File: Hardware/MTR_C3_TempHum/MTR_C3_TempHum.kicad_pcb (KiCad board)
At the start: 4 copper layers, 75 x 19 mm, 6 parts, among them IC1 ESP32-C3-MINI-1-H4, IC2 BQ25170DSGR, IC3 TLV76733DRVR, IC4 DHT22, J1 USB_C_Receptacle_USB2.0

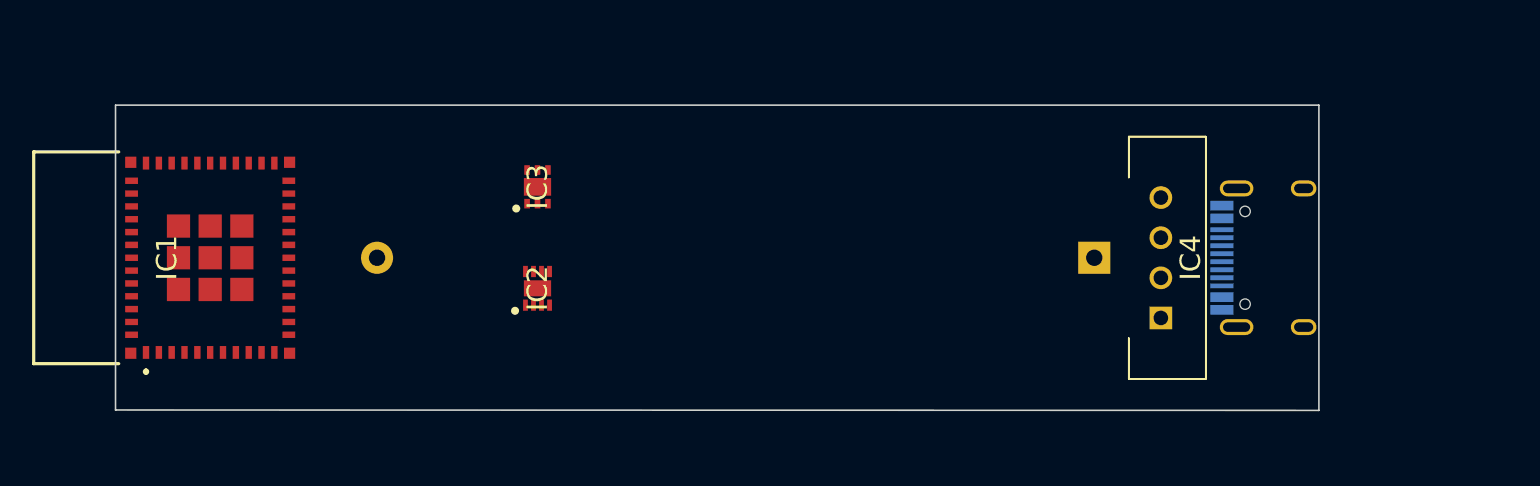
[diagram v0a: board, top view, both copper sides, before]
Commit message: REV 0.1
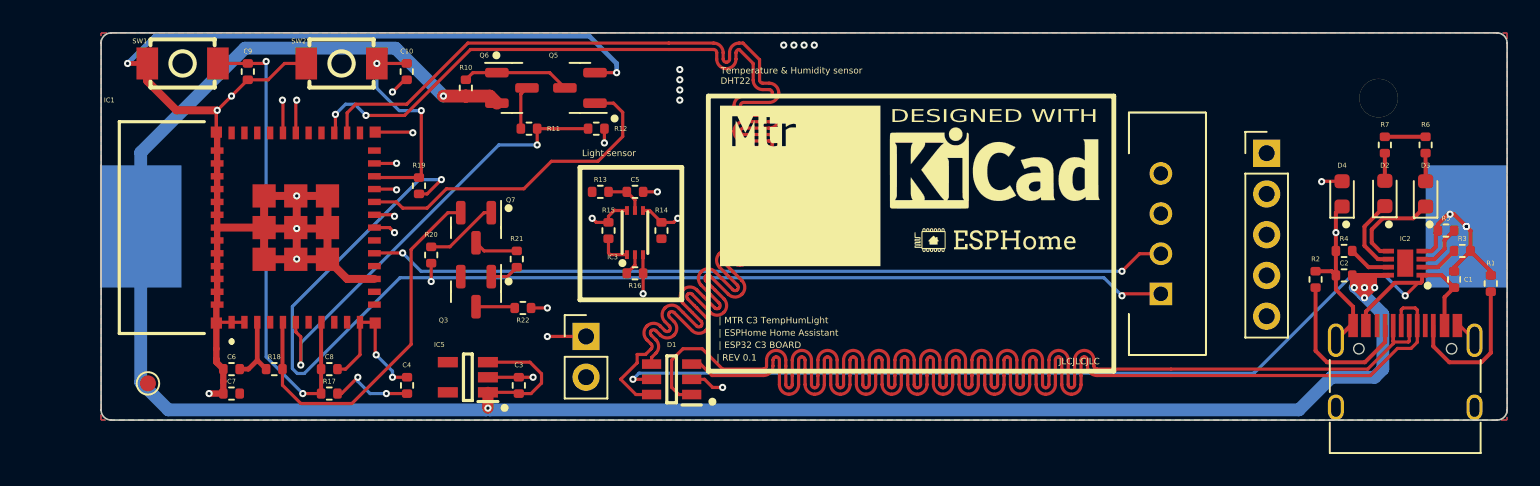
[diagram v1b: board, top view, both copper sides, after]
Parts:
- added ?: , clipboard:4e852f44-b39c-41c1-9906-6824c0cbc5c7, F.Cu at (62.7, 28.7)
- added ?: , clipboard:4e852f44-b39c-41c1-9906-6824c0cbc5c7, F.Cu at (63.2, 50.7)
- added ?: , clipboard:4e852f44-b39c-41c1-9906-6824c0cbc5c7, F.Cu at (118.4, 39.2)
- added ?: , clipboard:4e852f44-b39c-41c1-9906-6824c0cbc5c7, F.Cu at (120.9, 39.2)
- added ?: , clipboard:4e852f44-b39c-41c1-9906-6824c0cbc5c7, F.Cu at (70.1, 32.6)
- added ?: , clipboard:4e852f44-b39c-41c1-9906-6824c0cbc5c7, F.Cu at (76.2, 50.3)
- added ?: , clipboard:4e852f44-b39c-41c1-9906-6824c0cbc5c7, F.Cu at (63.5, 42.8)
- added ?: , clipboard:907f2ce9-957e-4633-84d2-7c9ab30228eb, F.Cu at (98.7, 40.8)
- added ?: , clipboard:4e852f44-b39c-41c1-9906-6824c0cbc5c7, F.Cu at (63.5, 38.2)
- added ?: , clipboard:4e852f44-b39c-41c1-9906-6824c0cbc5c7, F.Cu at (115.7, 39.2)
- added C1: 1u, Resistor_SMD:R_0402_1005Metric, F.Cu at (122.4, 42.7)
- added C10: 0.1u, Resistor_SMD:R_0402_1005Metric, F.Cu at (57.1, 29.7)
- added C2: 1u, Resistor_SMD:R_0402_1005Metric, F.Cu at (115.6, 42.4)
- added C3: 1u, Resistor_SMD:R_0402_1005Metric, F.Cu at (64.1, 49.3)
- added C4: 1u, Resistor_SMD:R_0402_1005Metric, F.Cu at (57.2, 49.3)
- added C5: 0.1u, Resistor_SMD:R_0402_1005Metric, F.Cu at (71.4, 37.2)
- added C6: 10u, Resistor_SMD:R_0402_1005Metric, F.Cu at (46.2, 48.3)
- added C7: 10u, Resistor_SMD:R_0402_1005Metric, F.Cu at (46.2, 49.8)
- added C8: 1u, Resistor_SMD:R_0402_1005Metric, F.Cu at (52.3, 48.3)
- added C9: 0.1u, Resistor_SMD:R_0402_1005Metric, F.Cu at (47.2, 29.7)
- added D1: USBLC6-2SC6, SamacSys_Parts:SOT95P280X145-6N, F.Cu at (73.7, 48.9)
- added D2: Emerald, LED_SMD:LED_0603_1608Metric, F.Cu at (118.1, 37.3)
- added D3: Blue, LED_SMD:LED_0603_1608Metric, F.Cu at (120.7, 37.3)
- added D4: Red, LED_SMD:LED_0603_1608Metric, F.Cu at (115.4, 37.3)
- added G***: LOGO, logoMTR, F.Cu at (81.7, 36.8)
- added IC5: RT9080-33GJ5, SamacSys_Parts:SOT94P280X100-5N, F.Cu at (61.0, 48.8)
- added J2: Boot Option, PinHeader:PinHeader_1x02_P2.54mm_Vertical, F.Cu at (68.3, 46.2)
- added J4: B5B-XH-A_LF__SN_, PinHeader:PinHeader_1x05_P2.54mm_Vertical, F.Cu at (110.7, 34.8)
- added Q3: AO3401A, Package_TO_SOT_SMD:SOT-23, F.Cu at (61.5, 43.4)
- added Q5: AO3402, Package_TO_SOT_SMD:SOT-23, F.Cu at (67.9, 30.7)
- added Q6: AO3401A, Package_TO_SOT_SMD:SOT-23, F.Cu at (63.7, 30.7)
- added Q7: AO3402, Package_TO_SOT_SMD:SOT-23, F.Cu at (61.5, 39.4)
- added R1: 5k1, Resistor_SMD:R_0402_1005Metric, F.Cu at (124.7, 42.9)
- added R10: 100k, Resistor_SMD:R_0402_1005Metric, F.Cu at (60.8, 30.7)
- added R11: 100k, Resistor_SMD:R_0402_1005Metric, F.Cu at (64.8, 33.3)
- added R12: 100k, Resistor_SMD:R_0402_1005Metric, F.Cu at (69.0, 33.3)
- added R13: 1k, Resistor_SMD:R_0402_1005Metric, F.Cu at (69.2, 37.2)
- added R14: 4k7, Resistor_SMD:R_0402_1005Metric, F.Cu at (73.0, 39.6)
- added R15: 4k7, Resistor_SMD:R_0402_1005Metric, F.Cu at (69.7, 39.6)
- added R16: 1k, Resistor_SMD:R_0402_1005Metric, F.Cu at (71.4, 42.3)
- added R17: 10k, Resistor_SMD:R_0402_1005Metric, F.Cu at (52.3, 49.8)
- added R18: 10k, Resistor_SMD:R_0402_1005Metric, F.Cu at (48.9, 48.3)
- added R19: 10k, Resistor_SMD:R_0402_1005Metric, F.Cu at (57.9, 36.8)
- added R2: 5k1, Resistor_SMD:R_0402_1005Metric, F.Cu at (113.8, 42.7)
- added R20: 10k, Resistor_SMD:R_0402_1005Metric, F.Cu at (58.7, 41.1)
- added R21: 10k, Resistor_SMD:R_0402_1005Metric, F.Cu at (64.0, 41.4)
- added R22: 120, Resistor_SMD:R_0402_1005Metric, F.Cu at (64.4, 44.5)
- added R3: 430, Resistor_SMD:R_0402_1005Metric, F.Cu at (122.9, 40.9)
- added R4: 27k, Resistor_SMD:R_0402_1005Metric, F.Cu at (115.6, 40.9)
- added R5: 10k, Resistor_SMD:R_0402_1005Metric, F.Cu at (121.9, 39.6)
- added R6: 10k, Resistor_SMD:R_0402_1005Metric, F.Cu at (120.7, 34.3)
- added R7: 10k, Resistor_SMD:R_0402_1005Metric, F.Cu at (118.1, 34.3)
- added REF**: LOGO, Library:KiCad, B.Cu at (93.3, 35.7)
- added SW1: Reset, easyeda2kicad:SW-SMD_L4.0-W3.0-LS5.0, F.Cu at (43.2, 29.2)
- added SW2: Hard_reset, easyeda2kicad:SW-SMD_L4.0-W3.0-LS5.0, F.Cu at (53.1, 29.2)
- added TP1: TestPoint, TestPoint:TestPoint_Pad_D1.0mm, F.Cu at (41.0, 49.1)
- BT1: value Battery_Cell -> 3000mAh; footprint Battery:BatteryHolder_Keystone_2466_1xAAA -> easyeda2kicad:BATTERY-SMD_18650-1S-L77.1-W20.7-1
- IC3: value TLV76733DRVR -> BH1750FVI-TR; footprint SamacSys_Parts:SON65P200X200X80-7N -> SamacSys_Parts:WSOF6
- J1: value USB_C_Receptacle_USB2.0 -> Korean Hroparts Elec TYPE-C-31-M-12; moved to F.Cu
- moved IC2 54.1 mm to (119.4, 41.7), turned to 180 degrees
- moved BT1 18.2 mm to (81.9, 39.4), turned to 90 degrees
- moved J1 11.1 mm to (119.4, 49.6), turned to 0 degrees
- moved IC3 6.71 mm to (71.4, 39.8)
- moved IC1 5.66 mm to (50.2, 39.4)
- moved IC4 1.50 mm to (104.2, 43.6)
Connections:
- BT1 pad 1: unconnected-(BT1-+-Pad1) -> VBAT
- BT1 pad 2: unconnected-(BT1---Pad2) -> GND
- IC1 pad 1: unconnected-(IC1-GND_1-Pad1) -> GND
- IC1 pad 11: unconnected-(IC1-GND_3-Pad11) -> GND
- IC1 pad 14: unconnected-(IC1-GND_4-Pad14) -> GND
- IC1 pad 16: unconnected-(IC1-IO10-Pad16) -> DHT22_DATA
- IC1 pad 18: unconnected-(IC1-IO4-Pad18) -> SDA
- IC1 pad 19: unconnected-(IC1-IO5-Pad19) -> SCL
- IC1 pad 2: unconnected-(IC1-GND_2-Pad2) -> GND
- IC1 pad 20: unconnected-(IC1-IO6-Pad20) -> EN_lvl_BAT
- IC1 pad 21: unconnected-(IC1-IO7-Pad21) -> GPIO7
- IC1 pad 22: unconnected-(IC1-IO8-Pad22) -> Hard_reset
- IC1 pad 23: unconnected-(IC1-IO9-Pad23) -> GPIO9
- IC1 pad 26: unconnected-(IC1-IO18-Pad26) -> USB_D-
- IC1 pad 27: unconnected-(IC1-IO19-Pad27) -> USB_D+
- IC1 pad 3: unconnected-(IC1-3V3-Pad3) -> +3.3V
- IC1 pad 30: unconnected-(IC1-RXD0-Pad30) -> UART_RX
- IC1 pad 31: unconnected-(IC1-TXD0-Pad31) -> UART_TX
- IC1 pad 36: unconnected-(IC1-GND_5-Pad36) -> GND
- IC1 pad 37: unconnected-(IC1-GND_6-Pad37) -> GND
- IC1 pad 38: unconnected-(IC1-GND_7-Pad38) -> GND
- IC1 pad 39: unconnected-(IC1-GND_8-Pad39) -> GND
- IC1 pad 40: unconnected-(IC1-GND_9-Pad40) -> GND
- IC1 pad 41: unconnected-(IC1-GND_10-Pad41) -> GND
- IC1 pad 42: unconnected-(IC1-GND_11-Pad42) -> GND
- IC1 pad 43: unconnected-(IC1-GND_12-Pad43) -> GND
- IC1 pad 44: unconnected-(IC1-GND_13-Pad44) -> GND
- IC1 pad 45: unconnected-(IC1-GND_14-Pad45) -> GND
- IC1 pad 46: unconnected-(IC1-GND_15-Pad46) -> GND
- IC1 pad 47: unconnected-(IC1-GND_16-Pad47) -> GND
- IC1 pad 48: unconnected-(IC1-GND_17-Pad48) -> GND
- IC1 pad 49: unconnected-(IC1-GND_18-Pad49) -> GND
- IC1 pad 5: unconnected-(IC1-IO2-Pad5) -> BAT_lvl_LED
- IC1 pad 50: unconnected-(IC1-GND_19-Pad50) -> GND
- IC1 pad 51: unconnected-(IC1-GND_20-Pad51) -> GND
- IC1 pad 52: unconnected-(IC1-GND_21-Pad52) -> GND
- IC1 pad 53: unconnected-(IC1-GND_22-Pad53) -> GND
- IC1 pad 54: unconnected-(IC1-GND_23-Pad54) -> GND
- IC1 pad 55: unconnected-(IC1-GND_24-Pad55) -> GND
- IC1 pad 56: unconnected-(IC1-GND_25-Pad56) -> GND
- IC1 pad 57: unconnected-(IC1-GND_26-Pad57) -> GND
- IC1 pad 58: unconnected-(IC1-GND_27-Pad58) -> GND
- IC1 pad 59: unconnected-(IC1-GND_28-Pad59) -> GND
- IC1 pad 6: unconnected-(IC1-IO3-Pad6) -> ADC_lvl_BAT
- IC1 pad 60: unconnected-(IC1-GND_29-Pad60) -> GND
- IC1 pad 61: unconnected-(IC1-GND_30-Pad61) -> GND
- IC1 pad 8: unconnected-(IC1-EN-Pad8) -> EN
- IC2 pad 1: unconnected-(IC2-IN-Pad1) -> VBUS
- IC2 pad 2: unconnected-(IC2-ISET-Pad2) -> Net-(IC2-ISET)
- IC2 pad 3: unconnected-(IC2-TS-Pad3) -> Net-(IC2-TS)
- IC2 pad 4: unconnected-(IC2-GND-Pad4) -> GND
- IC2 pad 5: unconnected-(IC2-STAT-Pad5) -> Net-(D3-K)
- IC2 pad 6: unconnected-(IC2-~{PG}-Pad6) -> Net-(D2-K)
- IC2 pad 7: unconnected-(IC2-VSET-Pad7) -> Net-(IC2-VSET)
- IC2 pad 8: unconnected-(IC2-OUT-Pad8) -> VBAT
- IC3 pad 1: unconnected-(IC3-OUT-Pad1) -> +3.3V
- IC3 pad 2: unconnected-(IC3-SNS-Pad2) -> Net-(IC3-ADDR)
- IC3 pad 3: unconnected-(IC3-GND_1-Pad3) -> GND
- IC3 pad 4: unconnected-(IC3-EN-Pad4) -> SDA
- IC3 pad 5: unconnected-(IC3-GND_2-Pad5) -> Net-(IC3-DVI)
- IC3 pad 6: unconnected-(IC3-IN-Pad6) -> SCL
- IC4 pad 1: unconnected-(IC4-VDD-Pad1) -> +3.3V
- IC4 pad 2: unconnected-(IC4-DATA-Pad2) -> DHT22_DATA
- IC4 pad 4: unconnected-(IC4-GND-Pad4) -> GND
- J1 pad A1: Net-(J1-GND-PadA1) -> GND
- J1 pad A12: Net-(J1-GND-PadA1) -> GND
- J1 pad A4: Net-(J1-VBUS-PadA4) -> VBUS
- J1 pad A5: unconnected-(J1-CC1-PadA5) -> Net-(J1-CC1)
- J1 pad A6: unconnected-(J1-D+-PadA6) -> /D+
- J1 pad A7: unconnected-(J1-D--PadA7) -> /D-
- J1 pad A9: Net-(J1-VBUS-PadA4) -> VBUS
- J1 pad B1: Net-(J1-GND-PadA1) -> GND
- J1 pad B12: Net-(J1-GND-PadA1) -> GND
- J1 pad B4: Net-(J1-VBUS-PadA4) -> VBUS
- J1 pad B5: unconnected-(J1-CC2-PadB5) -> Net-(J1-CC2)
- J1 pad B6: unconnected-(J1-D+-PadB6) -> /D+
- J1 pad B7: unconnected-(J1-D--PadB7) -> /D-
- J1 pad B9: Net-(J1-VBUS-PadA4) -> VBUS
- J1 pad S1: unconnected-(J1-SHIELD-PadS1) -> GND
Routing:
- net VBAT: track 0.00 -> 154.5 mm, vias 0 -> 6
- net GND: track 0.00 -> 147.6 mm, vias 0 -> 21
- net +3.3V: track 0.00 -> 126.1 mm, vias 0 -> 13
- net /D-: track 0.00 -> 102.2 mm
- net /D+: track 0.00 -> 98.9 mm
- net USB_D+: track 0.00 -> 96.1 mm, vias 0 -> 2
- net USB_D-: track 0.00 -> 91.5 mm
- net UART_TX: track 0.00 -> 68.8 mm, vias 0 -> 1
- net UART_RX: track 0.00 -> 64.9 mm, vias 0 -> 1
- net VBUS: track 0.00 -> 64.2 mm, vias 0 -> 2
- net GPIO7: track 0.00 -> 56.6 mm, vias 0 -> 1
- net Net-(D4-A): track 0.00 -> 53.8 mm, vias 0 -> 2
- net DHT22_DATA: track 0.00 -> 50.0 mm, vias 0 -> 2
- net EN: track 0.00 -> 30.3 mm, vias 0 -> 2
- net ADC_lvl_BAT: track 0.00 -> 28.2 mm, vias 0 -> 2
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- added copper zone on F.Cu, net +3.3V
- added copper zone on B.Cu, net GND
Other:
- board size 75 x 19 mm -> 87.6 x 24.1 mm
- board text added: "JLCJLCJLC"
- board text added: "Light sensor"
- board text added: "Temperature & Humidity sensor DHT22"
- board text added: "| ESP32 C3 BOARD"
- board text added: "| ESPHome Home Assistant"
- board text added: "| MTR C3 TempHumLight"
- board text added: "| REV 0.1"
